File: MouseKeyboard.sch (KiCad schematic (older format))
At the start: 12 parts

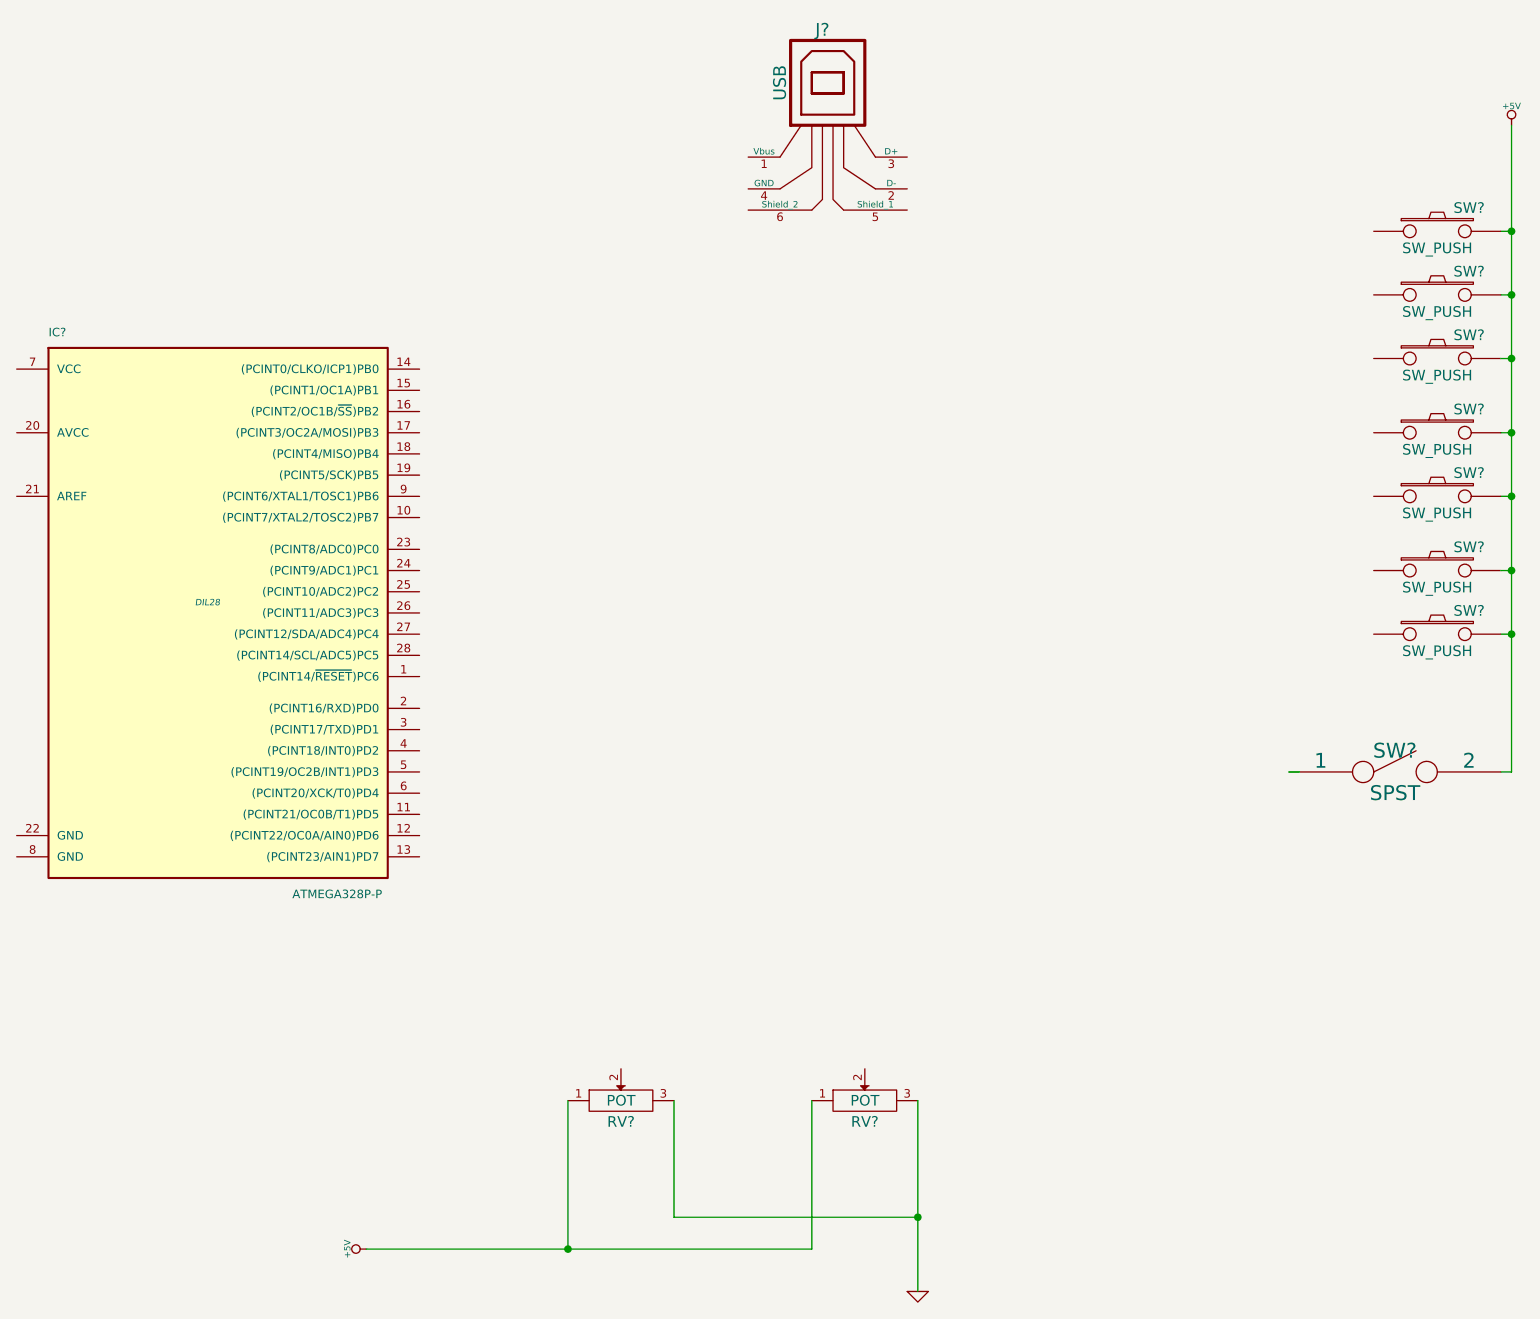
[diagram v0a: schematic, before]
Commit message: More Wires
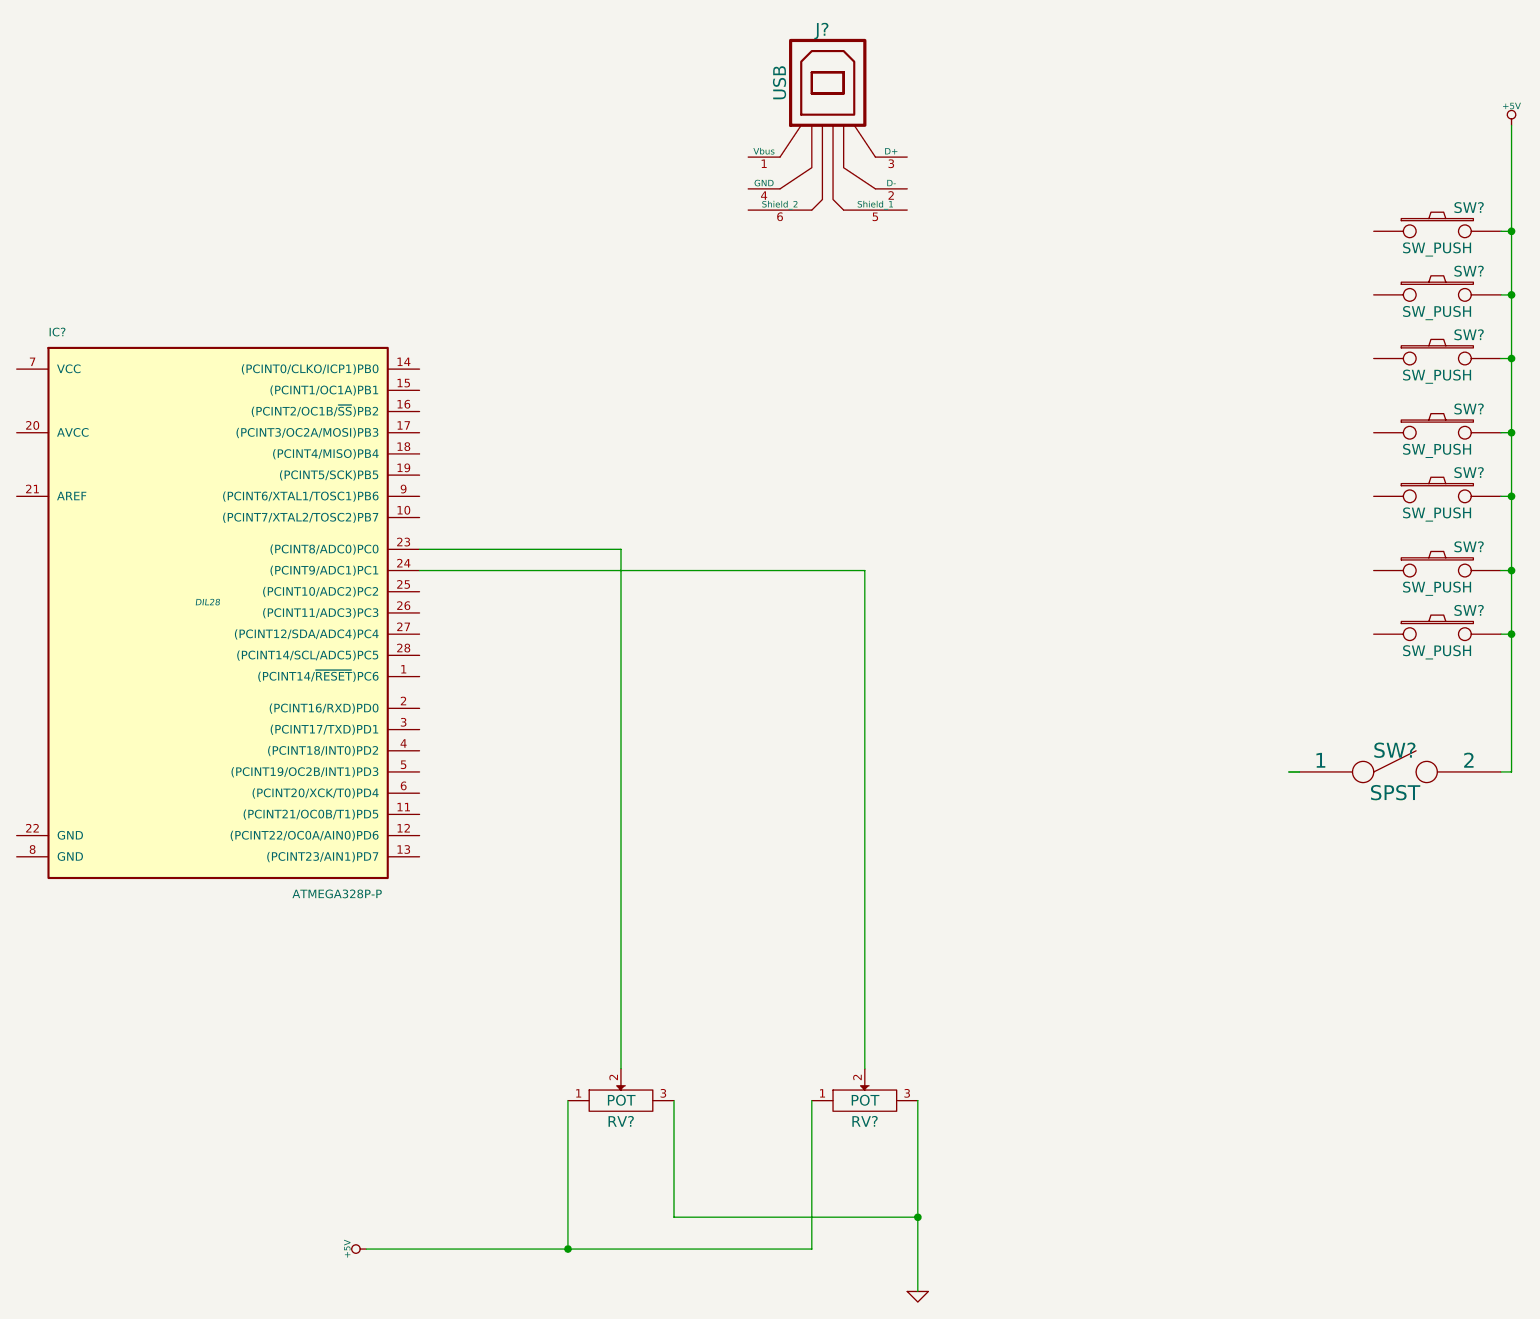
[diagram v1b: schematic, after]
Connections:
- wire segments 25 -> 20
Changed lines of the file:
@@
 $EndComp
 Wire Wire Line
-	3250 6550 4200 6550
-Wire Wire Line
-	4200 6550 5350 6550
+	3250 6550 5350 6550
 Wire Wire Line
 	4200 6550 4200 5850
@@
 Connection ~ 4200 6550
 Wire Wire Line
-	5850 6750 5850 6400
-Wire Wire Line
-	5850 6400 5850 5850
+	5850 5850 5850 6750
 Wire Wire Line
 	4700 5850 4700 6400
@@
 	8600 1750 8650 1750
 Wire Wire Line
-	8650 1250 8650 1750
-Wire Wire Line
-	8650 1750 8650 2050
-Wire Wire Line
-	8650 2050 8650 2350
-Wire Wire Line
-	8650 2350 8650 2700
-Wire Wire Line
-	8650 2700 8650 3000
-Wire Wire Line
-	8650 3000 8650 3350
-Wire Wire Line
-	8650 3350 8650 3650
-Wire Wire Line
-	8650 3650 8650 4300
+	8650 1250 8650 4300
 Wire Wire Line
 	8650 2050 8600 2050
@@
 	1    0    0    -1
 $EndComp
+Wire Wire Line
+	4450 5700 4450 3250
+Wire Wire Line
+	4450 3250 3500 3250
+Wire Wire Line
+	5600 5700 5600 3350
+Wire Wire Line
+	5600 3350 3500 3350
 $EndSCHEMATC
